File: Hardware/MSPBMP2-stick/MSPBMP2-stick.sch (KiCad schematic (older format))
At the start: 54 parts, among them J1 48037-0001, J2 JTAG, J3 SWD, U1 STM32L432KBU6, U2 LD1117AG-33-AB3-A-R, U3 AD8531ARTZ, U4 TXS0108EPWR, Y1 32768

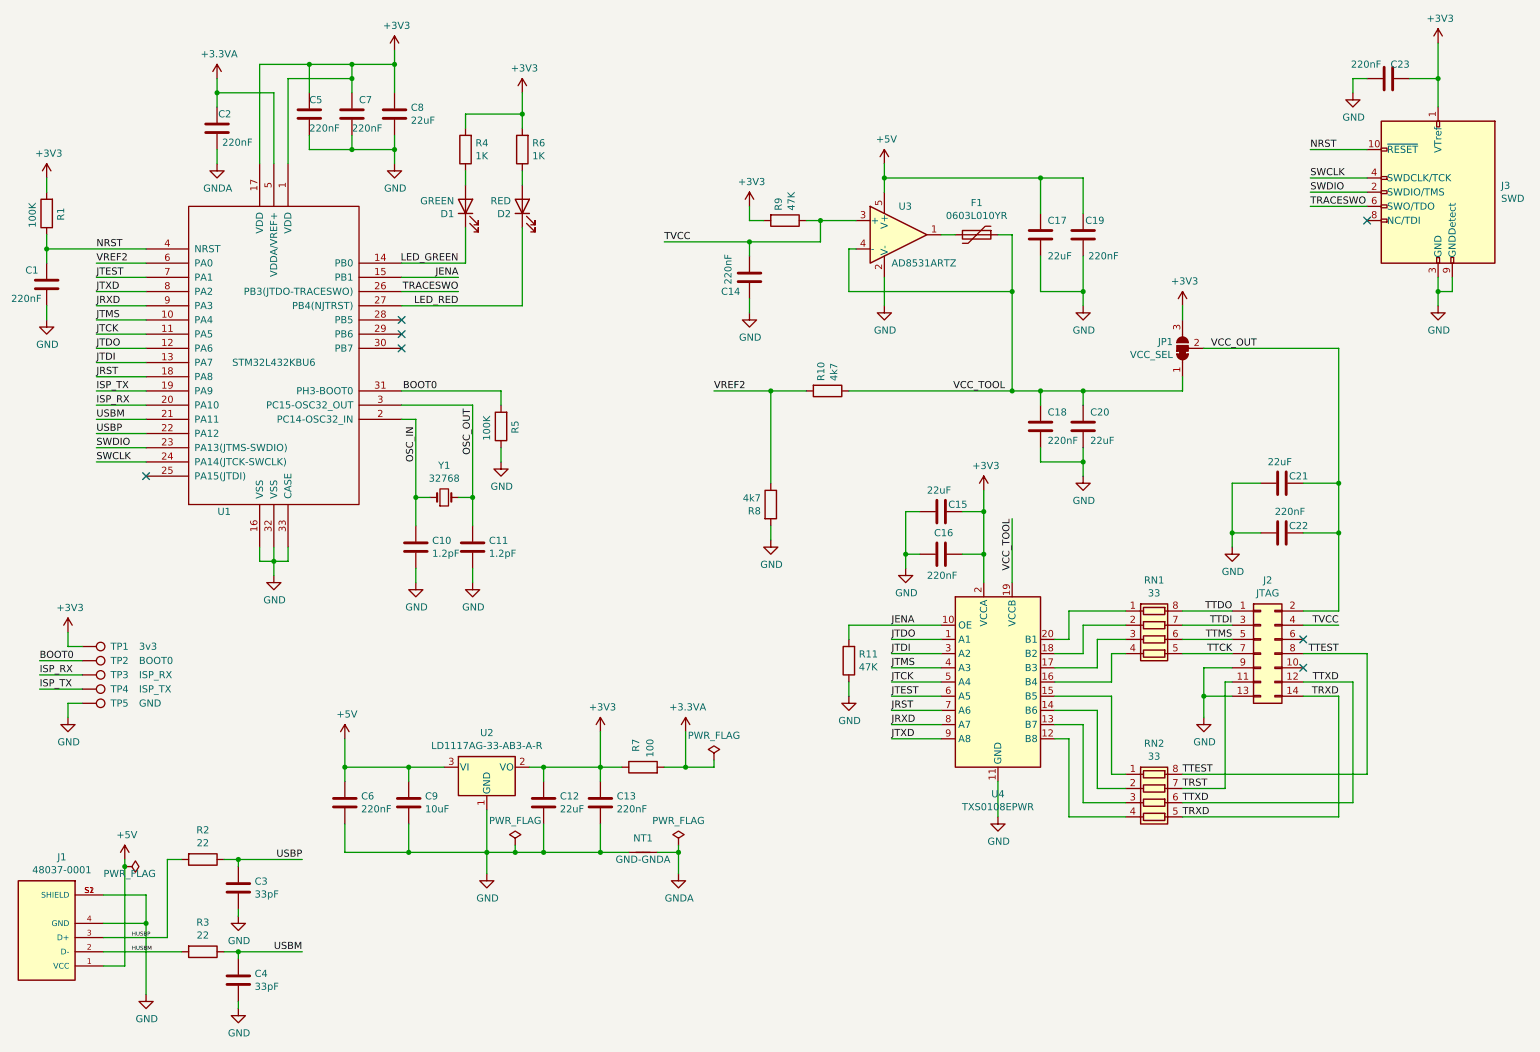
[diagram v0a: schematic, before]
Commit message: Schema update of PCB-Stick
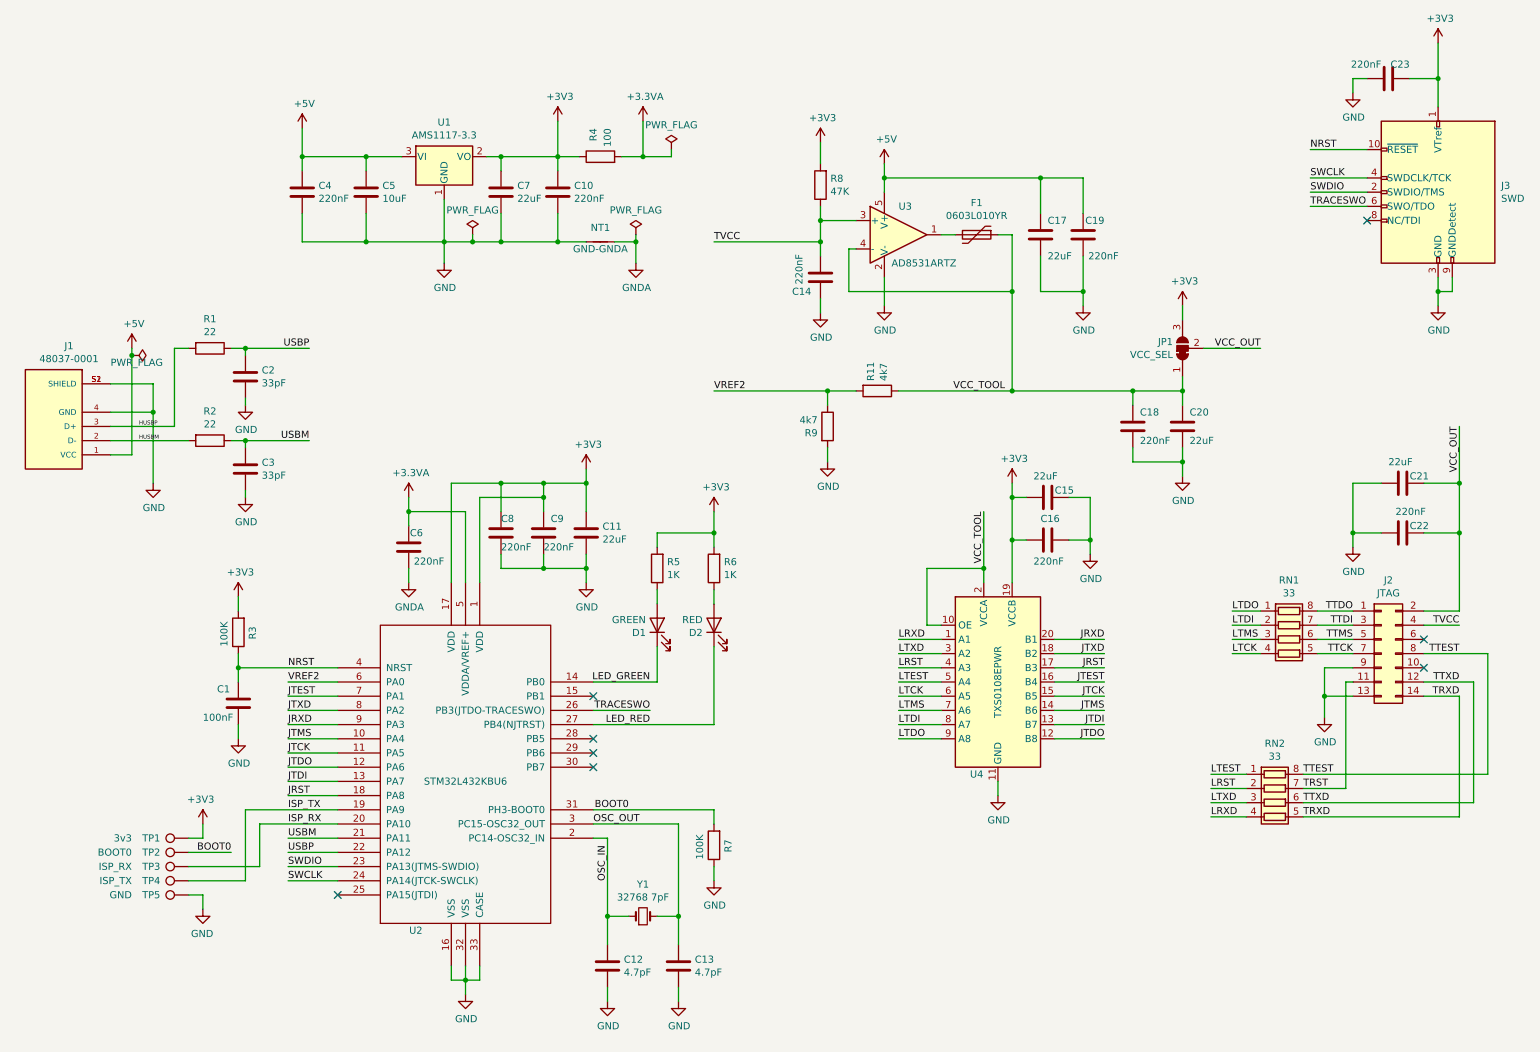
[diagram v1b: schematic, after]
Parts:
- removed R11: 47K, Resistor_SMD:R_0402_1005Metric_Pad0.72x0.64mm_HandSolder, symbol Device:R
- C1: value 220nF -> 100nF; Descr Multilayer Ceramic Capacitors MLCC - SMD/SMT 220nF 16V 0402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 -> 100nF ±10% 16V X7R 0402 Multilayer Ceramic Capacitors MLCC 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; LCSC C16772 -> C1525
- C12: renamed from C10; value 1.2pF -> 4.7pF; Descr 1.5pF ±0.25pF 50V C0G 0402 Multilayer Ceramic Capacitors ML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 -> 4.7pF ±0.25pF 50V C0G 0402 Multilayer Ceramic Capacitors ML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; LCSC C1552 -> C1569
- C13: renamed from C11; value 1.2pF -> 4.7pF; Descr 1.5pF ±0.25pF 50V C0G 0402 Multilayer Ceramic Capacitors ML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 -> 4.7pF ±0.25pF 50V C0G 0402 Multilayer Ceramic Capacitors ML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; LCSC C1552 -> C1569
- RN1, RN2: footprint Resistor_SMD:R_Array_Convex_4x0402 -> LocalLib:R_Array_Convex_4x0402_hand_soldered
- U1: renamed from U2; value LD1117AG-33-AB3-A-R -> AMS1117-3.3; Descr Fixed 15V 3.3V 1.3V @ 1A SOT-89(SOT-89-3) Dropout Regulator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 -> Fixed 10V 3.3V 1.3V @ 1A SOT-89 Dropout Regulators(LDO) RoHS; LCSC C81768 -> C347256
- U2: renamed from U1; Descr (none) -> 32-Bit FLASH ARM® Cortex®-M4 80MHz 1.71V ~ 3.6V UFQFPN-32 S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; LCSC (none) -> C94784
- U3: footprint Package_TO_SOT_SMD:TSOT-23-5_HandSoldering -> Package_TO_SOT_SMD:SOT-23-5_HandSoldering
- Y1: value 32768 -> 32768 7pF; Descr 32.768KHz ±20ppm 12.5pF 70kΩ 3215 SMD Crystal Resonators Ro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 -> 32.768KHz ±20ppm 7pF 70kΩ SMD-3215_2P SMD Crystal Resonator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; LCSC C271654 -> C97604
- renumbered C13 to C10, C8 to C11, C3 to C2, C4 to C3, C6 to C4, C9 to C5, C2 to C6, C12 to C7, C5 to C8, C7 to C9, R2 to R1, R10 to R11, R3 to R2, R1 to R3, R7 to R4, R4 to R5, R5 to R7, R9 to R8, R8 to R9
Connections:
- net +3V3: now also C15.2, C16.2, U4.19 (VCCB); no longer C15.1, C16.1, U4.2 (VCCA)
- net GND: now also C15.1, C16.1; no longer C15.2, C16.2
- net JRST: now also U4.17 (B3); no longer U4.7 (A6)
- net JRXD: now also U4.20 (B1); no longer U4.8 (A7)
- net JTCK: now also U4.15 (B5); no longer U4.5 (A4)
- net JTDI: now also U4.13 (B7); no longer U4.3 (A2)
- net JTDO: now also U4.12 (B8); no longer U4.1 (A1)
- net JTEST: now also U4.16 (B4); no longer U4.6 (A5)
- net JTMS: now also U4.14 (B6); no longer U4.4 (A3)
- net JTXD: now also U4.18 (B2); no longer U4.9 (A8)
- net VCC_TOOL: now also U4.10 (OE), U4.2 (VCCA); no longer U4.19 (VCCB)
- net LRXD: now reaches RN2.4 (R4.1)
- net LRXD: now also U4.1 (A1); no longer U4.12 (B8)
- net LTXD: now reaches RN2.3 (R3.1)
- net LTXD: now also U4.3 (A2); no longer U4.13 (B7)
- net LRST: now reaches RN2.2 (R2.1)
- net LRST: now also U4.4 (A3); no longer U4.14 (B6)
- net LTEST: now reaches RN2.1 (R1.1)
- net LTEST: now also U4.5 (A4); no longer U4.15 (B5)
- net LTCK: now reaches RN1.4 (R4.1)
- net LTCK: now also U4.6 (A5); no longer U4.16 (B4)
- net LTMS: now reaches RN1.3 (R3.1)
- net LTMS: now also U4.7 (A6); no longer U4.17 (B3)
- net LTDI: now reaches RN1.2 (R2.1)
- net LTDI: now also U4.8 (A7); no longer U4.18 (B2)
- net LTDO: now reaches RN1.1 (R1.1)
- net LTDO: now also U4.9 (A8); no longer U4.20 (B1)
- net JENA: no longer names the net of U2.15 (PB1)
- net JENA: no longer U4.10 (OE)
- no-connect marks 7 -> 8
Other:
- moved on the sheet: C1, C10, C11, C12, C13, C14, C15, C16, C18, C2, C20, C21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
